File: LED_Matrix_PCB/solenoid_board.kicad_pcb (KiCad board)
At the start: 2 copper layers, 185 x 130 mm, 97 parts, among them J2 MCU_LEFT_LEGS, J3 MCU_RIGHT_LEGS

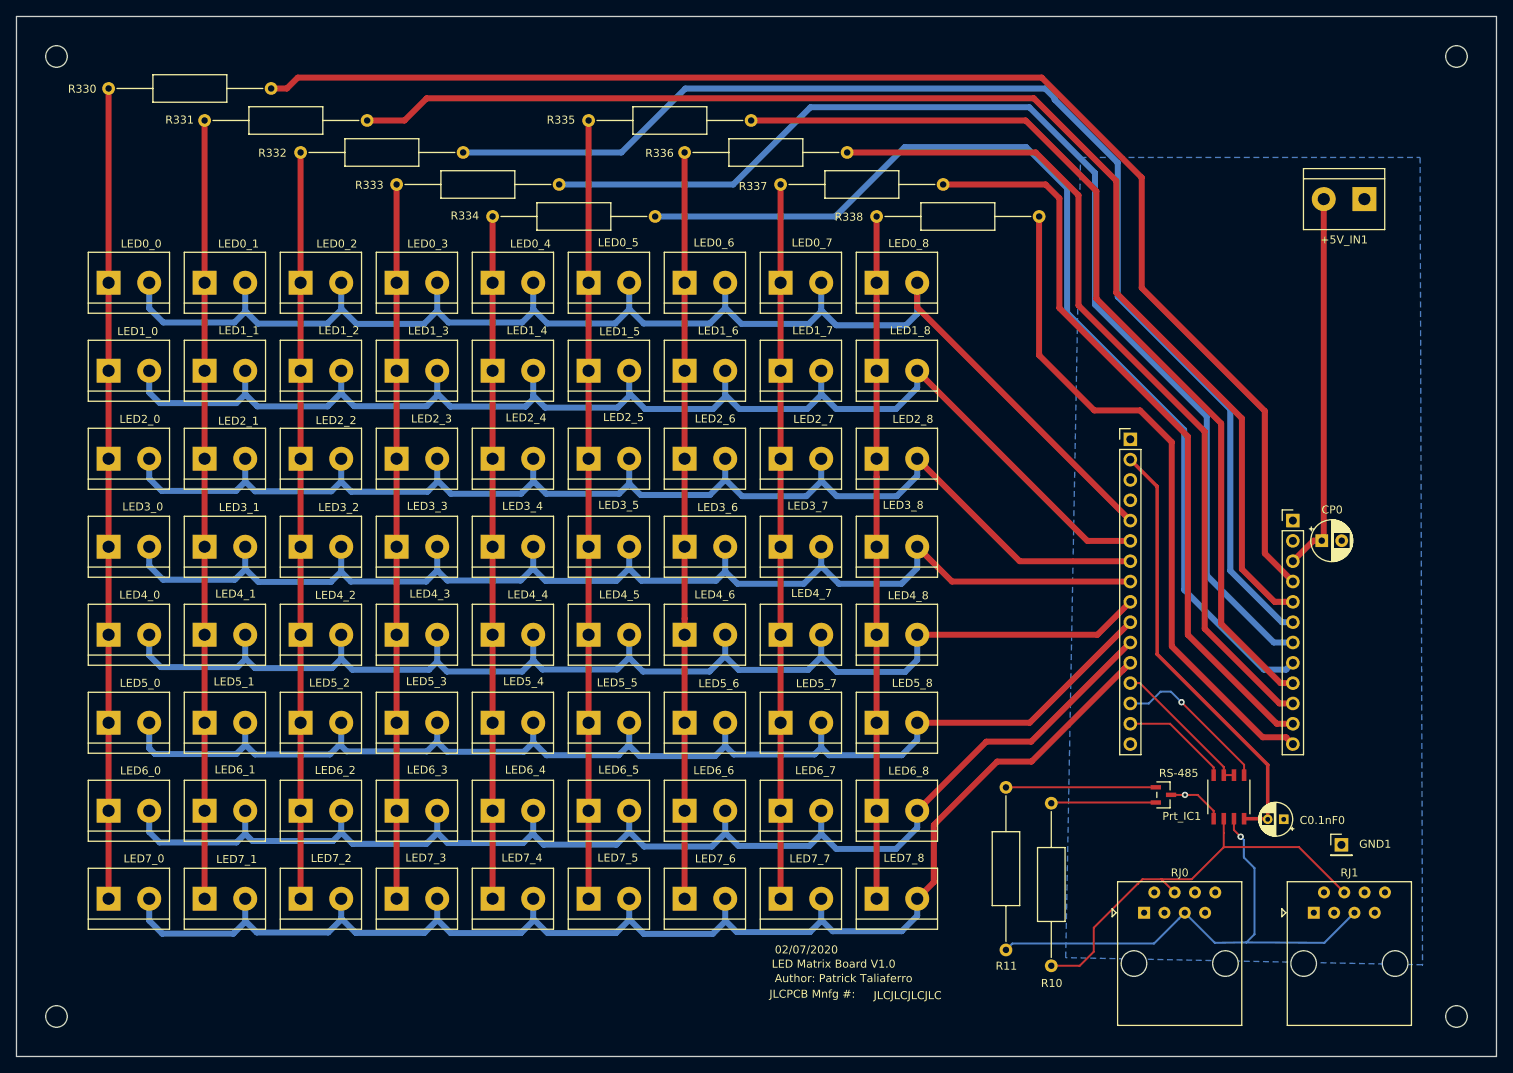
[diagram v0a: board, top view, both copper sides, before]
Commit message: Forgot to close files before pushing.
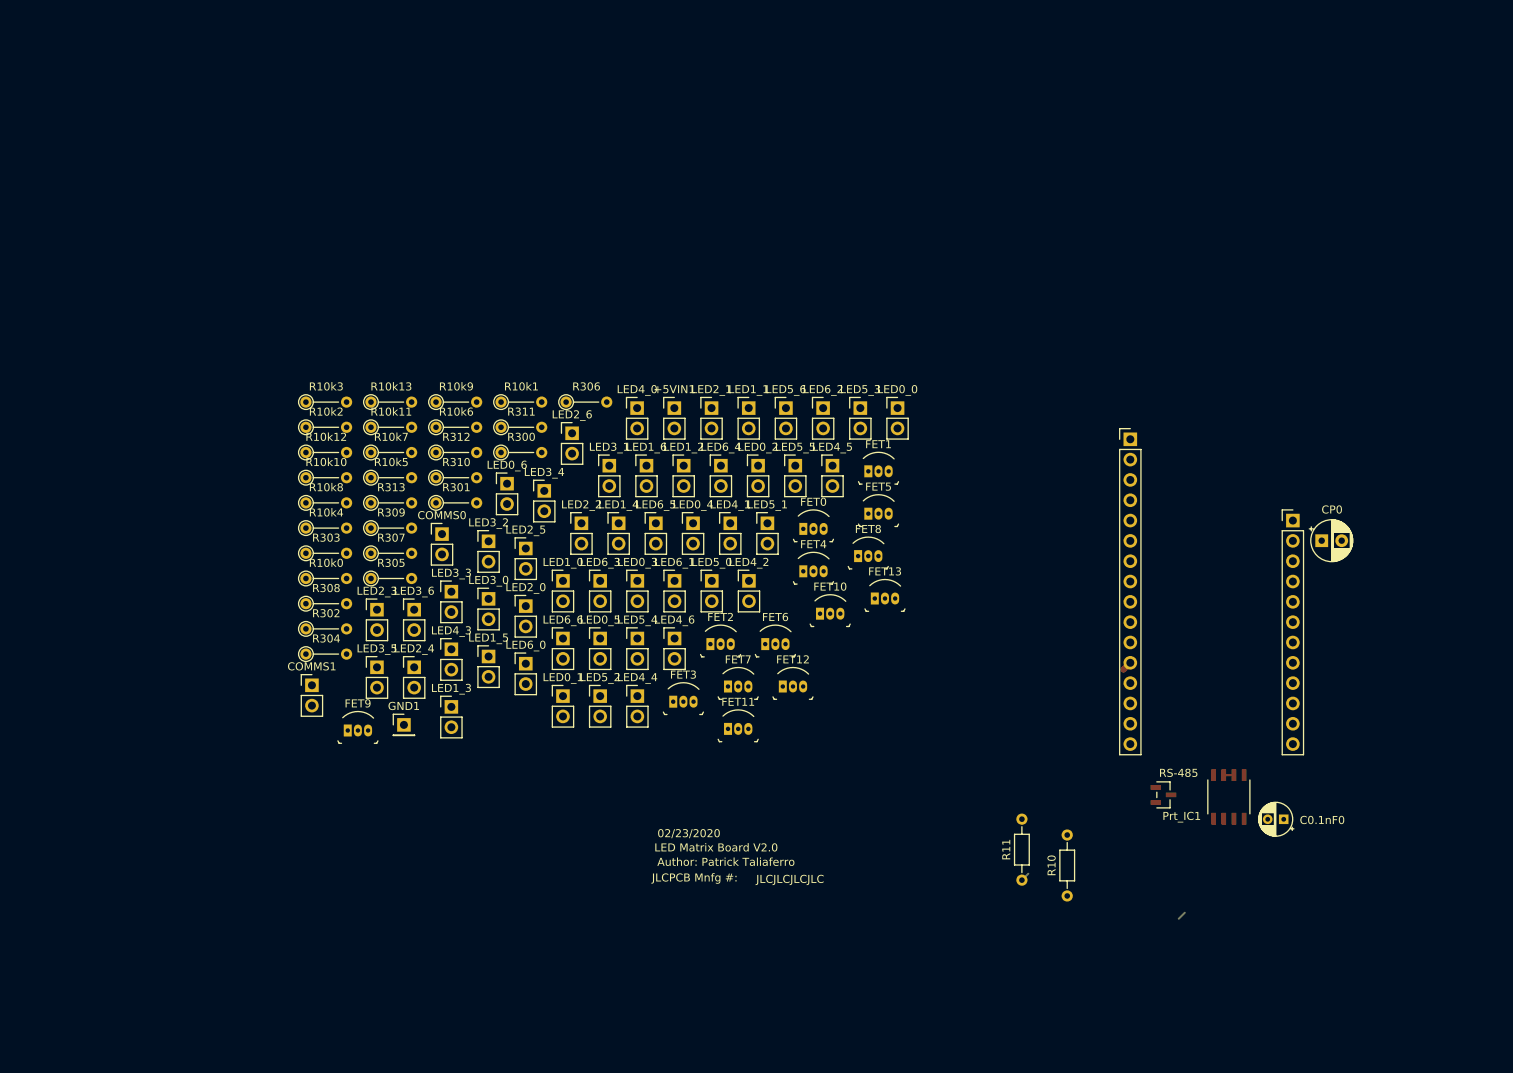
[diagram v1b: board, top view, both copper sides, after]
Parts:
- removed +5V_IN1: MCU_PWR_Supply, TerminalBlock:TerminalBlock_bornier-2_P5.08mm
- removed LED0_7, LED0_8, LED1_7, LED1_8, LED2_7, LED2_8, LED3_7, LED3_8, LED4_7, LED4_8, LED5_7, LED5_8, LED6_7, LED6_8, LED7_0, LED7_1, LED7_2, LED7_3, LED7_4, LED7_5, LED7_6, LED7_7, LED7_8: Screw-terminal, TerminalBlock:TerminalBlock_bornier-2_P5.08mm
- removed R330, R331, R332: 330, Resistor_THT:R_Axial_DIN0309_L9.0mm_D3.2mm_P20.32mm_Horizontal
- removed R333, R334, R335, R336, R337, R338: R, Resistor_THT:R_Axial_DIN0309_L9.0mm_D3.2mm_P20.32mm_Horizontal
- removed REF** (x4): MountingHole_2.7mm_M2.5, MountingHole:MountingHole_2.7mm_M2.5
- removed RJ0, RJ1: RJ45, Connector_RJ:RJ45_Amphenol_54602-x08_Horizontal
- added +5VIN1: Conn_01x02, Connector_PinHeader_2.54mm:PinHeader_1x02_P2.54mm_Vertical, F.Cu at (132.2, 74.0)
- added COMMS0: Conn_01x02, Connector_PinHeader_2.54mm:PinHeader_1x02_P2.54mm_Vertical, F.Cu at (103.2, 89.7)
- added COMMS1: Conn_01x02, Connector_PinHeader_2.54mm:PinHeader_1x02_P2.54mm_Vertical, F.Cu at (86.9, 108.6)
- added FET0: 2N7000, digikey-footprints:TO-92-3, F.Cu at (148.4, 89.1)
- added FET1: 2N7000, digikey-footprints:TO-92-3, F.Cu at (156.5, 81.9)
- added FET10: 2N7000, digikey-footprints:TO-92-3, F.Cu at (150.4, 99.7)
- added FET11: 2N7000, digikey-footprints:TO-92-3, F.Cu at (138.9, 114.1)
- added FET12: 2N7000, digikey-footprints:TO-92-3, F.Cu at (145.8, 108.8)
- added FET13: 2N7000, digikey-footprints:TO-92-3, F.Cu at (157.3, 97.8)
- added FET2: 2N7000, digikey-footprints:TO-92-3, F.Cu at (136.7, 103.5)
- added FET3: 2N7000, digikey-footprints:TO-92-3, F.Cu at (132.1, 110.7)
- added FET4: 2N7000, digikey-footprints:TO-92-3, F.Cu at (148.4, 94.4)
- added FET5: 2N7000, digikey-footprints:TO-92-3, F.Cu at (156.5, 87.2)
- added FET6: 2N7000, digikey-footprints:TO-92-3, F.Cu at (143.6, 103.5)
- added FET7: 2N7000, digikey-footprints:TO-92-3, F.Cu at (138.9, 108.8)
- added FET8: 2N7000, digikey-footprints:TO-92-3, F.Cu at (155.2, 92.5)
- added FET9: 2N7000, digikey-footprints:TO-92-3, F.Cu at (91.4, 114.3)
- added R10k0: 10k, Resistor_THT:R_Axial_DIN0204_L3.6mm_D1.6mm_P5.08mm_Vertical, F.Cu at (86.2, 95.3)
- added R10k1: 10k, Resistor_THT:R_Axial_DIN0204_L3.6mm_D1.6mm_P5.08mm_Vertical, F.Cu at (110.6, 73.2)
- added R10k10: 10k, Resistor_THT:R_Axial_DIN0204_L3.6mm_D1.6mm_P5.08mm_Vertical, F.Cu at (86.2, 82.7)
- added R10k11: 10k, Resistor_THT:R_Axial_DIN0204_L3.6mm_D1.6mm_P5.08mm_Vertical, F.Cu at (94.3, 76.4)
- added R10k12: 10k, Resistor_THT:R_Axial_DIN0204_L3.6mm_D1.6mm_P5.08mm_Vertical, F.Cu at (86.2, 79.5)
- added R10k13: 10k, Resistor_THT:R_Axial_DIN0204_L3.6mm_D1.6mm_P5.08mm_Vertical, F.Cu at (94.3, 73.2)
- added R10k2: 10k, Resistor_THT:R_Axial_DIN0204_L3.6mm_D1.6mm_P5.08mm_Vertical, F.Cu at (86.2, 76.4)
- added R10k3: 10k, Resistor_THT:R_Axial_DIN0204_L3.6mm_D1.6mm_P5.08mm_Vertical, F.Cu at (86.2, 73.2)
- added R10k4: 10k, Resistor_THT:R_Axial_DIN0204_L3.6mm_D1.6mm_P5.08mm_Vertical, F.Cu at (86.2, 89.0)
- added R10k5: 10k, Resistor_THT:R_Axial_DIN0204_L3.6mm_D1.6mm_P5.08mm_Vertical, F.Cu at (94.3, 82.7)
- added R10k6: 10k, Resistor_THT:R_Axial_DIN0204_L3.6mm_D1.6mm_P5.08mm_Vertical, F.Cu at (102.4, 76.4)
- added R10k7: 10k, Resistor_THT:R_Axial_DIN0204_L3.6mm_D1.6mm_P5.08mm_Vertical, F.Cu at (94.3, 79.5)
- added R10k8: 10k, Resistor_THT:R_Axial_DIN0204_L3.6mm_D1.6mm_P5.08mm_Vertical, F.Cu at (86.2, 85.8)
- added R10k9: 10k, Resistor_THT:R_Axial_DIN0204_L3.6mm_D1.6mm_P5.08mm_Vertical, F.Cu at (102.4, 73.2)
- added R300: 300, Resistor_THT:R_Axial_DIN0204_L3.6mm_D1.6mm_P5.08mm_Vertical, F.Cu at (110.6, 79.5)
- added R301: 300, Resistor_THT:R_Axial_DIN0204_L3.6mm_D1.6mm_P5.08mm_Vertical, F.Cu at (102.4, 85.8)
- added R302: 300, Resistor_THT:R_Axial_DIN0204_L3.6mm_D1.6mm_P5.08mm_Vertical, F.Cu at (86.2, 101.6)
- added R303: 300, Resistor_THT:R_Axial_DIN0204_L3.6mm_D1.6mm_P5.08mm_Vertical, F.Cu at (86.2, 92.1)
- added R304: 300, Resistor_THT:R_Axial_DIN0204_L3.6mm_D1.6mm_P5.08mm_Vertical, F.Cu at (86.2, 104.7)
- added R305: 300, Resistor_THT:R_Axial_DIN0204_L3.6mm_D1.6mm_P5.08mm_Vertical, F.Cu at (94.3, 95.3)
- added R306: 300, Resistor_THT:R_Axial_DIN0204_L3.6mm_D1.6mm_P5.08mm_Vertical, F.Cu at (118.7, 73.2)
- added R307: 300, Resistor_THT:R_Axial_DIN0204_L3.6mm_D1.6mm_P5.08mm_Vertical, F.Cu at (94.3, 92.1)
- added R308: 300, Resistor_THT:R_Axial_DIN0204_L3.6mm_D1.6mm_P5.08mm_Vertical, F.Cu at (86.2, 98.4)
- added R309: 300, Resistor_THT:R_Axial_DIN0204_L3.6mm_D1.6mm_P5.08mm_Vertical, F.Cu at (94.3, 89.0)
- added R310: 300, Resistor_THT:R_Axial_DIN0204_L3.6mm_D1.6mm_P5.08mm_Vertical, F.Cu at (102.4, 82.7)
- added R311: 300, Resistor_THT:R_Axial_DIN0204_L3.6mm_D1.6mm_P5.08mm_Vertical, F.Cu at (110.6, 76.4)
- added R312: 300, Resistor_THT:R_Axial_DIN0204_L3.6mm_D1.6mm_P5.08mm_Vertical, F.Cu at (102.4, 79.5)
- added R313: 300, Resistor_THT:R_Axial_DIN0204_L3.6mm_D1.6mm_P5.08mm_Vertical, F.Cu at (94.3, 85.8)
- GND1: value Conn_01x01_Male -> Conn_01x01
- LED0_0, LED0_1, LED0_2, LED0_3, LED0_4, LED0_5, LED0_6, LED1_0, LED1_1, LED1_2, LED1_3, LED1_4, LED1_5, LED1_6, LED2_0, LED2_1, LED2_2, LED2_3, LED2_4, LED2_5, LED2_6, LED3_0, LED3_1, LED3_2, LED3_3, LED3_4, LED3_5, LED3_6, LED4_0, LED4_1, LED4_2, LED4_3, LED4_4, LED4_5, LED4_6, LED5_0, LED5_1, LED5_2, LED5_3, LED5_4, LED5_5, LED5_6, LED6_0, LED6_1, LED6_2, LED6_3, LED6_4, LED6_5, LED6_6: value Screw-terminal -> Conn_01x02; footprint TerminalBlock:TerminalBlock_bornier-2_P5.08mm -> Connector_PinHeader_2.54mm:PinHeader_1x02_P2.54mm_Vertical
- R10, R11: footprint Resistor_THT:R_Axial_DIN0309_L9.0mm_D3.2mm_P20.32mm_Horizontal -> Resistor_THT:R_Axial_DIN0204_L3.6mm_D1.6mm_P7.62mm_Horizontal
- moved GND1 118.1 mm to (98.4, 113.6)
- moved LED0_0 99.9 mm to (160.1, 74.0)
- moved LED6_2 82.5 mm to (150.8, 74.0)
- moved LED5_0 77.5 mm to (136.9, 95.6)
- moved LED5_1 74.6 mm to (143.9, 88.4)
- moved LED4_0 71.9 mm to (127.6, 74.0)
- moved LED5_3 70.1 mm to (155.5, 74.0)
- moved LED0_1 68.4 mm to (118.3, 110.0)
- moved LED1_1 68.2 mm to (141.5, 74.0)
- moved LED4_1 67.2 mm to (139.2, 88.4)
- moved LED6_1 65.4 mm to (132.3, 95.6)
- moved LED2_1 63.7 mm to (136.9, 74.0)
- moved LED1_0 62.6 mm to (118.3, 95.6)
- moved LED0_2 61.6 mm to (142.7, 81.2)
- moved LED4_2 56.5 mm to (141.6, 95.6)
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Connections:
- net /RJ45_4 renamed /A
- net /RJ45_5 renamed /B
- J2 pad 11: /ROW6 -> (no net)
- J2 pad 12: /MOSI -> (no net)
- J3 pad 11: /SCL -> (no net)
- J3 pad 12: /SDA -> (no net)
- LED0_0 pad 2: /A0 -> /ROW0
- LED0_1 pad 2: /A0 -> /ROW0
- LED0_2 pad 2: /A0 -> /ROW0
- LED0_3 pad 2: /A0 -> /ROW0
- LED0_4 pad 2: /A0 -> /ROW0
- LED0_5 pad 2: /A0 -> /ROW0
- LED0_6 pad 2: /A0 -> /ROW0
- LED1_0 pad 2: /A1 -> /ROW1
- LED1_1 pad 2: /A1 -> /ROW1
- LED1_2 pad 2: /A1 -> /ROW1
- LED1_3 pad 2: /A1 -> /ROW1
- LED1_4 pad 2: /A1 -> /ROW1
- LED1_5 pad 2: /A1 -> /ROW1
- LED1_6 pad 2: /A1 -> /ROW1
- LED2_0 pad 2: /A2 -> /ROW2
- LED2_1 pad 2: /A2 -> /ROW2
- LED2_2 pad 2: /A2 -> /ROW2
- LED2_3 pad 2: /A2 -> /ROW2
- LED2_4 pad 2: /A2 -> /ROW2
- LED2_5 pad 2: /A2 -> /ROW2
- LED2_6 pad 2: /A2 -> /ROW2
- LED3_0 pad 2: /A3 -> /ROW3
- LED3_1 pad 2: /A3 -> /ROW3
- LED3_2 pad 2: /A3 -> /ROW3
- LED3_3 pad 2: /A3 -> /ROW3
- LED3_4 pad 2: /A3 -> /ROW3
- LED3_5 pad 2: /A3 -> /ROW3
- LED3_6 pad 2: /A3 -> /ROW3
- LED4_0 pad 2: /A4 -> /ROW4
- LED4_1 pad 2: /A4 -> /ROW4
- LED4_2 pad 2: /A4 -> /ROW4
- LED4_3 pad 2: /A4 -> /ROW4
- LED4_4 pad 2: /A4 -> /ROW4
- LED4_5 pad 2: /A4 -> /ROW4
- LED4_6 pad 2: /A4 -> /ROW4
- LED5_0 pad 2: /A5 -> /ROW5
- LED5_1 pad 2: /A5 -> /ROW5
- LED5_2 pad 2: /A5 -> /ROW5
- LED5_3 pad 2: /A5 -> /ROW5
- LED5_4 pad 2: /A5 -> /ROW5
- LED5_5 pad 2: /A5 -> /ROW5
- LED5_6 pad 2: /A5 -> /ROW5
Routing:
- net /A0: track 179.2 -> 0.00 mm
- net /MOSI: track 174.9 -> 0.00 mm
- net /D13: track 172.9 -> 0.00 mm
- net /A1: track 168.7 -> 0.00 mm
- net /ROW6: track 165.6 -> 0.00 mm
- net /A2: track 163.1 -> 0.00 mm
- net /D12: track 162.2 -> 0.00 mm
- net /A4: track 160.5 -> 0.00 mm
- net /A5: track 160.3 -> 0.00 mm
- net /A3: track 159.7 -> 0.00 mm
- net /D11: track 156.4 -> 0.00 mm
- net /D10: track 144.7 -> 0.00 mm
- net /D9: track 131.6 -> 0.00 mm
- net /D6: track 119.4 -> 0.00 mm
- net /D5: track 106.7 -> 0.00 mm
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- removed copper zone on B.Cu, net GND
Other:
- board outline removed
- board text added: "02/23/2020"
- board text added: "LED Matrix Board V2.0"
- board text removed: "02/07/2020"
- board text removed: "LED Matrix Board V1.0"
